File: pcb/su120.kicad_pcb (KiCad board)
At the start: 2 copper layers, 99.2 x 98.4 mm, 299 parts, among them J1 MJ-4PP-9, J2 Conn_01x03, J3 Conn_01x08, J4 Conn_01x08, J5 Conn_01x03, J6 MJ-4PP-9, SW1 SW_Push, SW10 SW_Push, SW11 SW_Push, SW12 SW_Push, SW13 SW_Push, SW14 SW_Push, SW15 SW_Push, SW16 SW_Push, SW17 SW_Push, SW18 SW_Push, SW19 SW_Push, SW2 SW_Push, SW20 SW_Push, SW21 SW_Push, SW3 SW_Push, SW4 SW_Push, SW5 SW_Push, SW6 SW_Push, SW7 SW_Push, SW8 SW_Push, SW9 SW_Push, U1 ProMicro

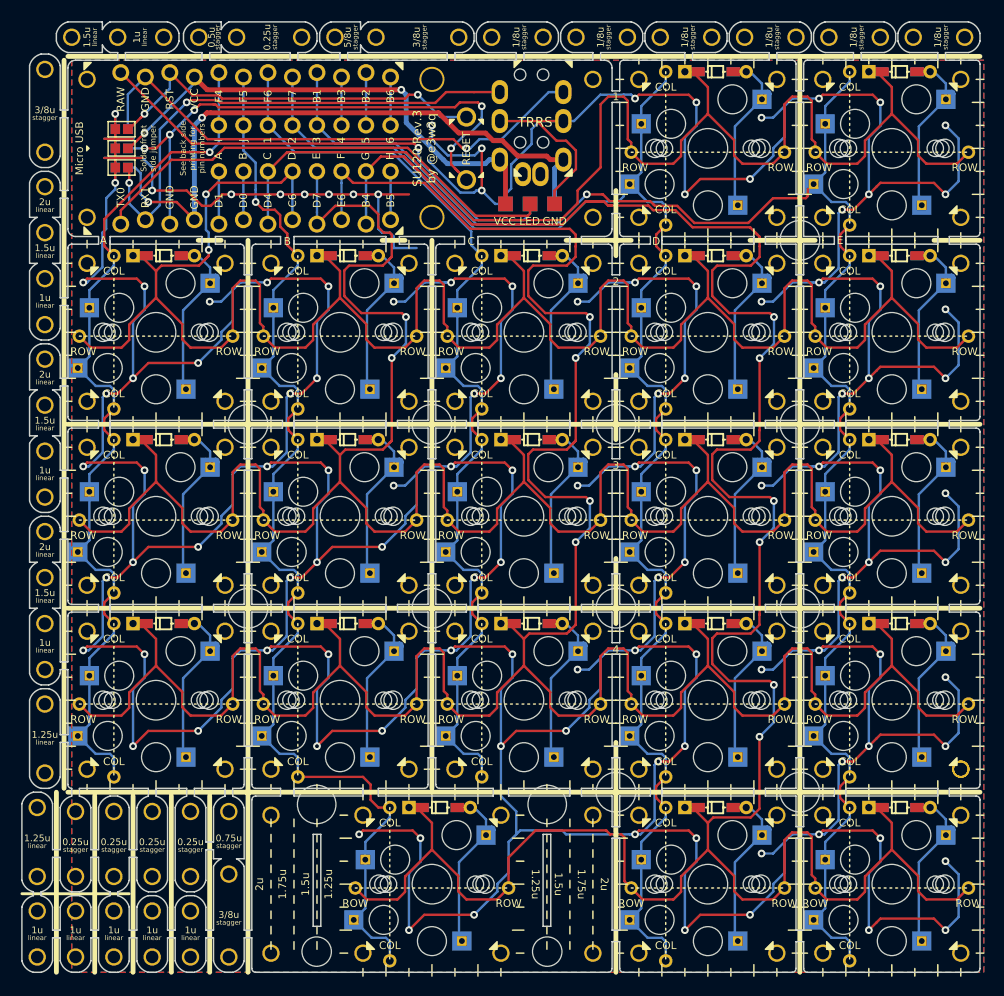
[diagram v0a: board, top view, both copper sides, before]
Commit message: Rev.4
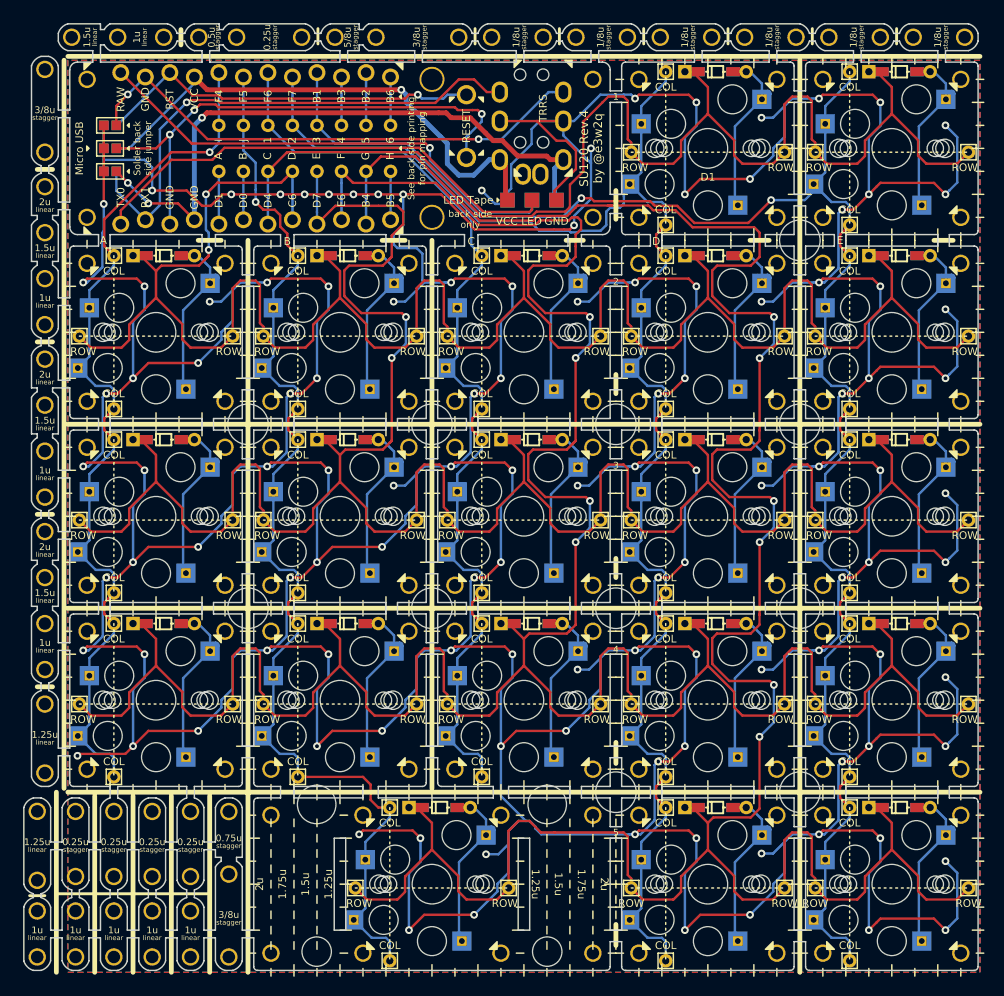
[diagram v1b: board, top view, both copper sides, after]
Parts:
- removed the ? at (118.3, 133.3)
- removed the ? at (99.2, 133.3)
- removed the ? at (118.3, 95.2)
- removed the ? at (99.2, 95.2)
- removed the ? at (80.2, 95.2)
- removed the ? at (61.1, 95.2)
- removed the ? at (61.1, 114.3)
- removed the ? at (80.2, 114.3)
- removed the ? at (99.2, 114.3)
- removed the ? at (118.3, 114.3)
- removed H157: MountingHole_Pad, #footprint:M1.4_tapping_Pad
- added ?: , #footprint:M2_spacer, F.Cu at (99.2, 133.4)
- added ?: , #footprint:M2_spacer, F.Cu at (118.3, 95.3)
- added ?: , #footprint:M2_spacer, F.Cu at (118.3, 133.4)
- added ?: , #footprint:M2_spacer, F.Cu at (118.3, 114.3)
- added ?: , #footprint:M2_spacer, F.Cu at (99.2, 114.3)
- added ?: , #footprint:M2_spacer, F.Cu at (80.2, 114.3)
- added ?: , #footprint:M2_spacer, F.Cu at (61.1, 114.3)
- added ?: , #footprint:M2_spacer, F.Cu at (61.1, 95.3)
- added ?: , #footprint:M2_spacer, F.Cu at (80.2, 95.3)
- added ?: , #footprint:M2_spacer, F.Cu at (99.2, 95.3)
- J3, J4: footprint #footprint:PinHeader_1x08_P2.54mm_Vertical -> #footprint:PinHeader_1x08_P2.54mm_Vertical_rev2
- JP1, JP4, JP6: moved to F.Cu
- JP2, JP3, JP5: moved to B.Cu
- moved SW18 2.31 mm to (83.7, 64.4)
- moved JP2 1.26 mm to (46.8, 69.1)
- moved JP6 1.26 mm to (46.8, 69.1)
- moved JP1 1.26 mm to (46.8, 64.3)
- moved JP3 1.26 mm to (46.8, 64.3)
- moved JP4 1.19 mm to (46.8, 66.7)
- moved JP5 1.19 mm to (46.8, 66.7)
- moved J2 0.44 mm to (88.0, 72.0)
- moved J5 0.44 mm to (93.1, 72.0)
- moved ? 0.40 mm to (39.3, 142.5)
- moved ? 0.40 mm to (39.3, 135.3)
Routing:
- net GND: track 978.4 -> 988.5 mm, vias 115 -> 117
- net reset1: track 59.2 -> 55.2 mm, vias 5 -> 3
- net Y3: track 262.4 -> 264.7 mm
- net Y4: track 307.3 -> 309.6 mm
- net dummyVCC: track 53.4 -> 55.7 mm, vias 2 -> 1
- net X4: track 161.5 -> 163.1 mm
- net dummydata: track 53.2 -> 54.4 mm, vias 2 -> 1
- net reset2: track 41.3 -> 40.1 mm, vias 2 -> 1
- net X3: track 101.5 -> 102.2 mm
- net data: track 55.8 -> 55.1 mm, vias 1 -> 2
- net Y1: track 137.2 -> 136.7 mm
- net X5: track 180.2 -> 180.5 mm, vias 1 -> 2
- net VCC: track 66.3 -> 66.1 mm, vias 2 -> 3
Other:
- board size 99.2 x 98.4 mm -> 98.8 x 98 mm
- board text added: "LED Tape"
- board text added: "SU120 Rev.4 by @e3w2q"
- board text added: "See back side printing for pin mapping"
- board text added: "Solder back side jumper"
- board text added: "back side only"
- board text removed: "SU120 Rev.3 by @e3w2q"
- board text removed: "See back side printing for pin numbers"
- board text removed: "Solder front side jumper"
